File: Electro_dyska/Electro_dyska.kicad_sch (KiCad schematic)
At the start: 4 parts

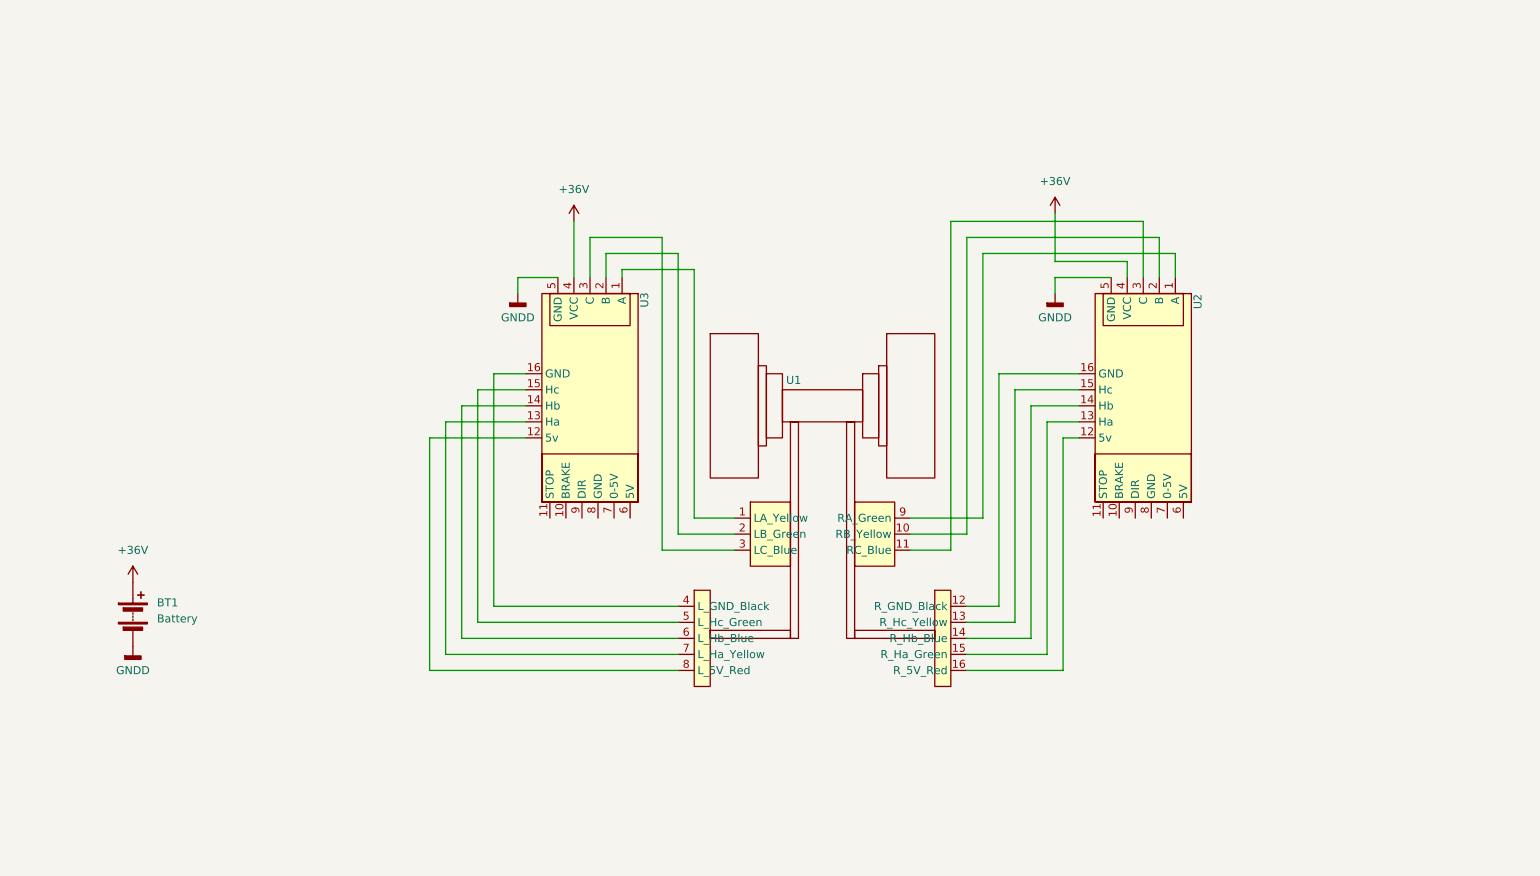
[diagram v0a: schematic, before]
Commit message: Updated schematics
Not finished
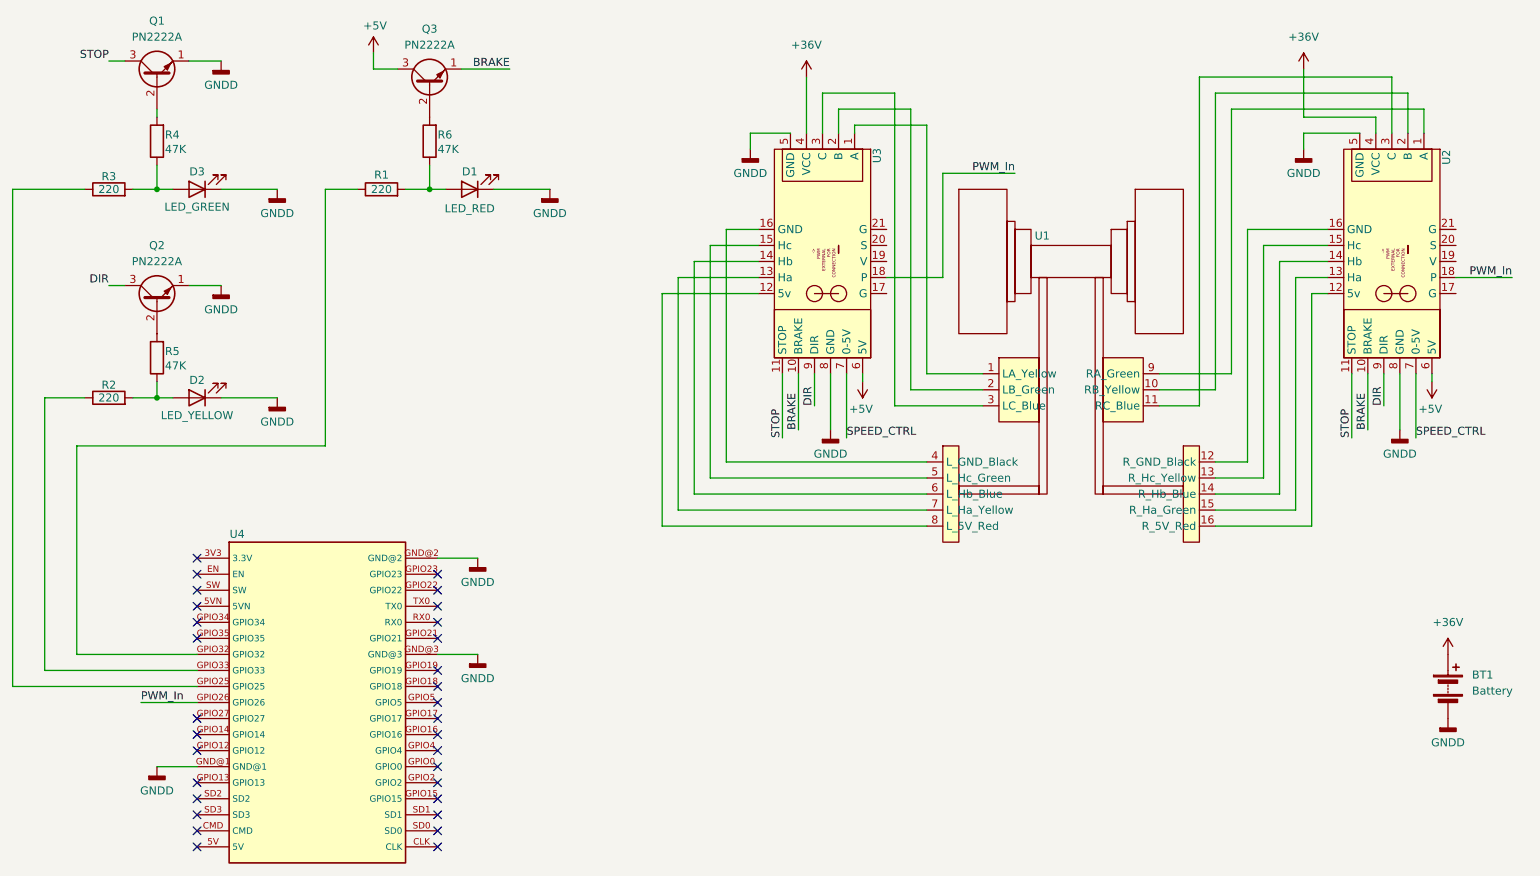
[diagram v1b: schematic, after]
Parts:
- added D1: LED_RED, symbol Device:LED
- added D2: LED_YELLOW, symbol Device:LED
- added D3: LED_GREEN, symbol Device:LED
- added Q1, Q2, Q3: PN2222A, Package_TO_SOT_THT:TO-92_Inline, symbol Transistor_BJT:PN2222A
- added R1, R2, R3: 220, symbol Device:R
- added R4, R5, R6: 47K, symbol Device:R
- added U4: ~, symbol ESP32S:ESP32S
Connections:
- net GNDD: now also U2.8 (GND), U3.8 (GND), D1.1 (K), D2.1 (K), D3.1 (K), Q1.1 (E), Q2.1 (E), U4.GND@1, U4.GND@2, U4.GND@3
- net BRAKE: now reaches U3.10 (BRAKE)
- net BRAKE: now also U2.10 (BRAKE), Q3.1 (E)
- net STOP: now reaches U3.11 (STOP)
- net STOP: now also U2.11 (STOP), Q1.3 (C)
- net +5V: now reaches U3.6 (5V)
- net +5V: now also U2.6 (5V), Q3.3 (C)
- net SPEED_CTRL: now reaches U3.7 (0-5V)
- net SPEED_CTRL: now also U2.7 (0-5V)
- net DIR: now reaches U3.9 (DIR)
- net DIR: now also U2.9 (DIR), Q2.3 (C)
- new net: D2.2 (A), R2.2, R5.1
- new net: D1.2 (A), R1.2, R6.1
- new net: Q3.2 (B), R6.2
- new net: D3.2 (A), R3.2, R4.1
- new net: R3.1, U4.GPIO25
- new net: R2.1, U4.GPIO33
- new net: R1.1, U4.GPIO32
- new net: Q1.2 (B), R4.2
- new net: Q2.2 (B), R5.2
- new net PWM_In: U2.18 (P), U3.18 (P), U4.GPIO26
- no-connect marks 0 -> 31
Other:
- moved on the sheet: BT1, U1
